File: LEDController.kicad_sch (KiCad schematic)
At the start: 15 parts, among them J1 3557-2, J11 TB002-500-04BE, J12 TB002-500-04BE, J16 3557-2, J17 TB002-500-04BE, J2 3557-2, J3 3557-2, J4 3557-2, J5 3557-2, J6 3557-2, J7 VP0265840000G, K1 J115F11CH5VDCS61.5U, Q1 BCX56,135

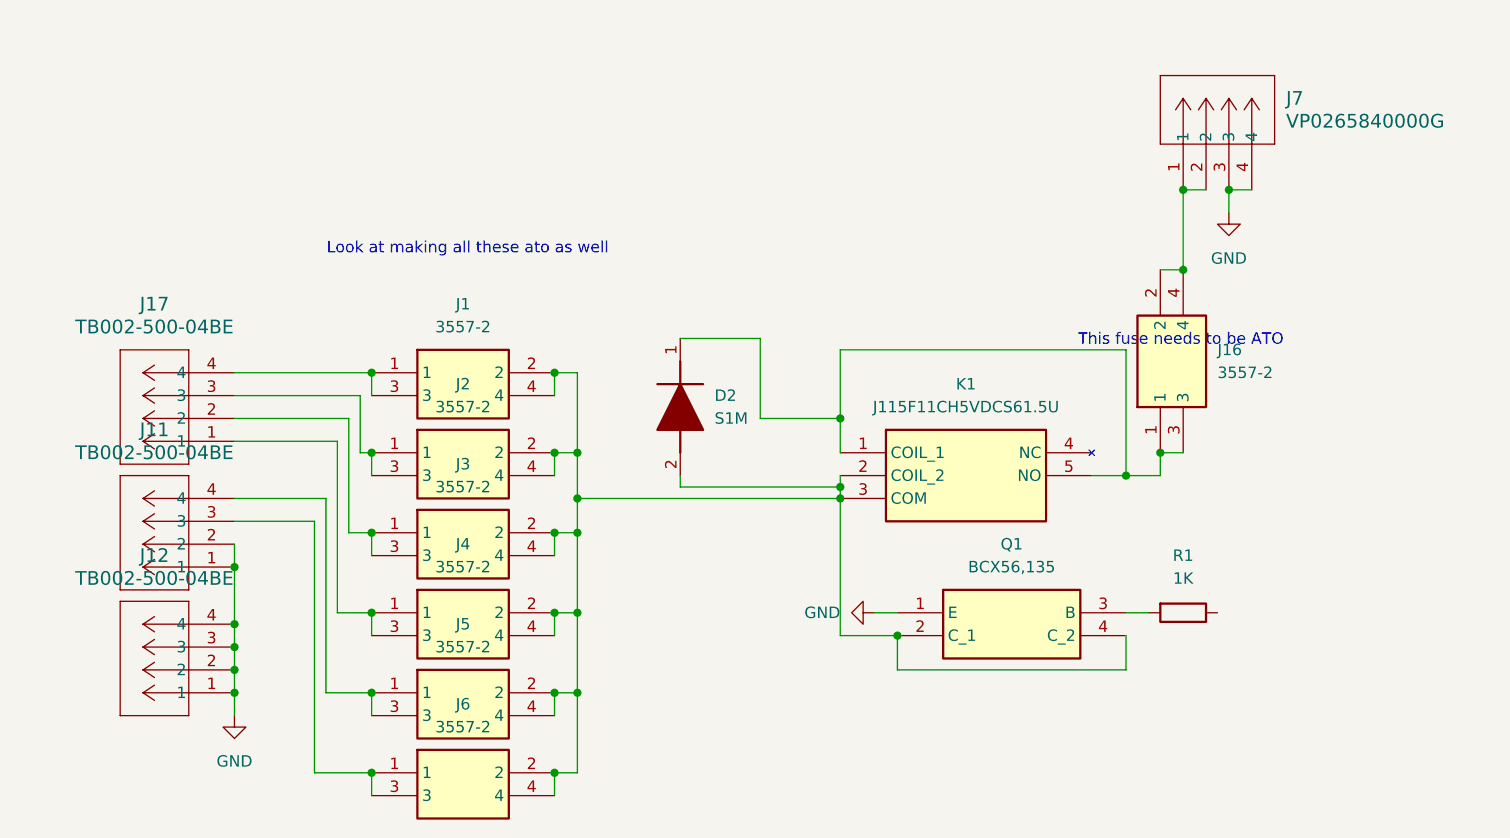
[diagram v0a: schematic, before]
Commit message: final schematic
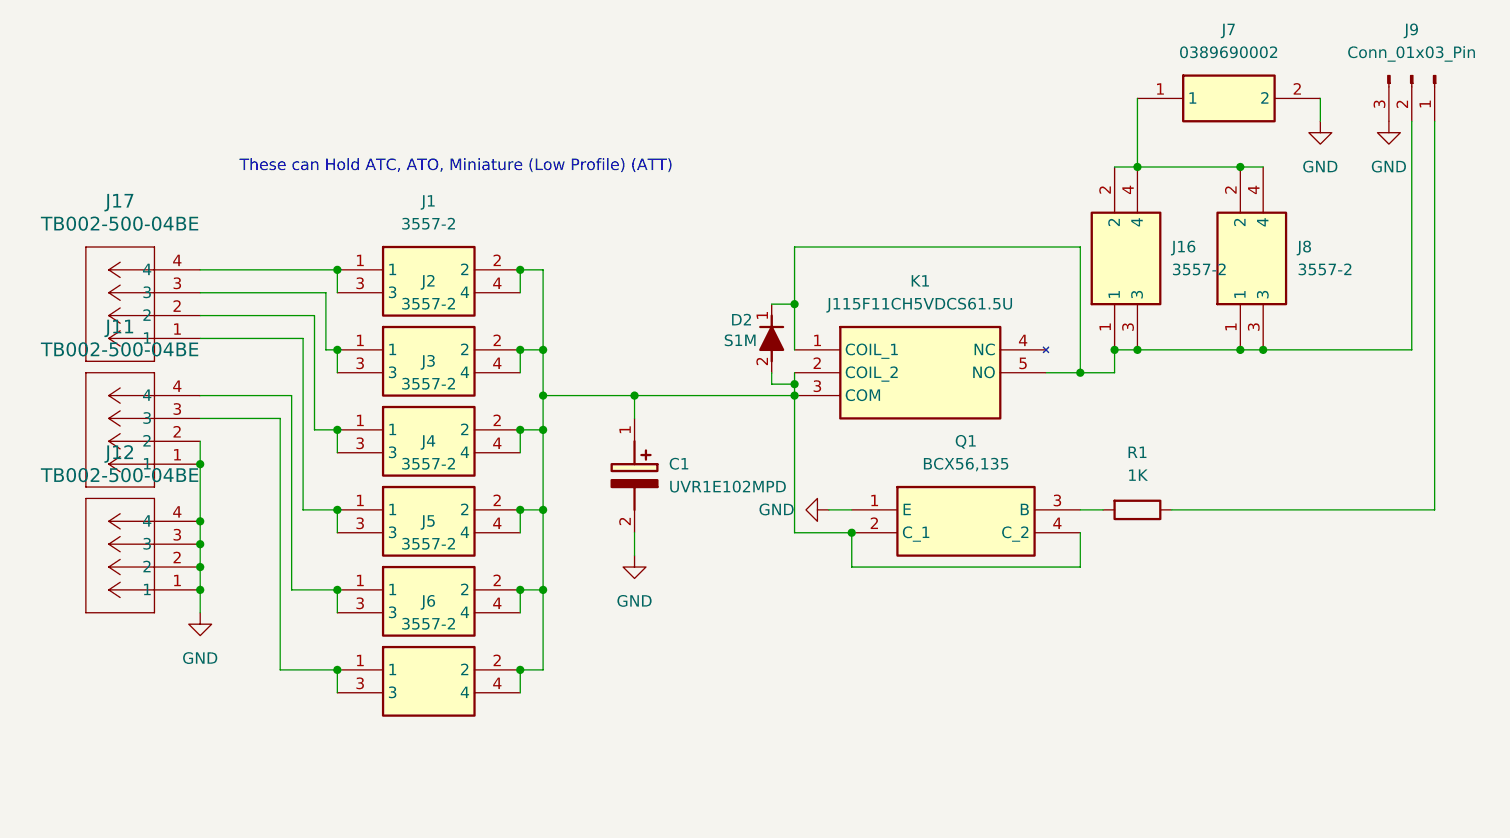
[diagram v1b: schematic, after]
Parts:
- removed J7: VP0265840000G, CONN04_VP026584_20P32X18P3_AMP, symbol SamacSys_Parts:VP0265840000G
- added C1: UVR1E102MPD, CAPPRD500W60D1025H2200, symbol SamacSys_Parts:UVR1E102MPD
- added J7: 0389690002, 0389690002, symbol SamacSys_Parts:0389690002
- added J8: 3557-2, 3557-2, symbol SamacSys_Parts:3557-2
- added J9: Conn_01x03_Pin, Connector_PinSocket_2.54mm:PinSocket_1x03_P2.54mm_Vertical, symbol Connector:Conn_01x03_Pin
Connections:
- net GND: now also C1.2 (-), J7.2, J9.3 (Pin_3)
- net at D2.2 (A), J1.2, J1.4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: now also C1.1 (+)
- net at D2.1 (K), J16.1, J16.3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: now also J8.1, J8.3, J9.2 (Pin_2)
- net at R1.1: now also J9.1 (Pin_1)
- net at J16.2, J16.4: now also J7.1, J8.2, J8.4
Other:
- note added: "These can Hold ATC, ATO, Miniature (Low Profile) (ATT)"
- note removed: "Look at making all these ato as well"
- note removed: "This fuse needs to be ATO"
- moved on the sheet: D2, J1, J11, J12, J16, J17, J2, J3, J4, J5, J6, K1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

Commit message: wip layout
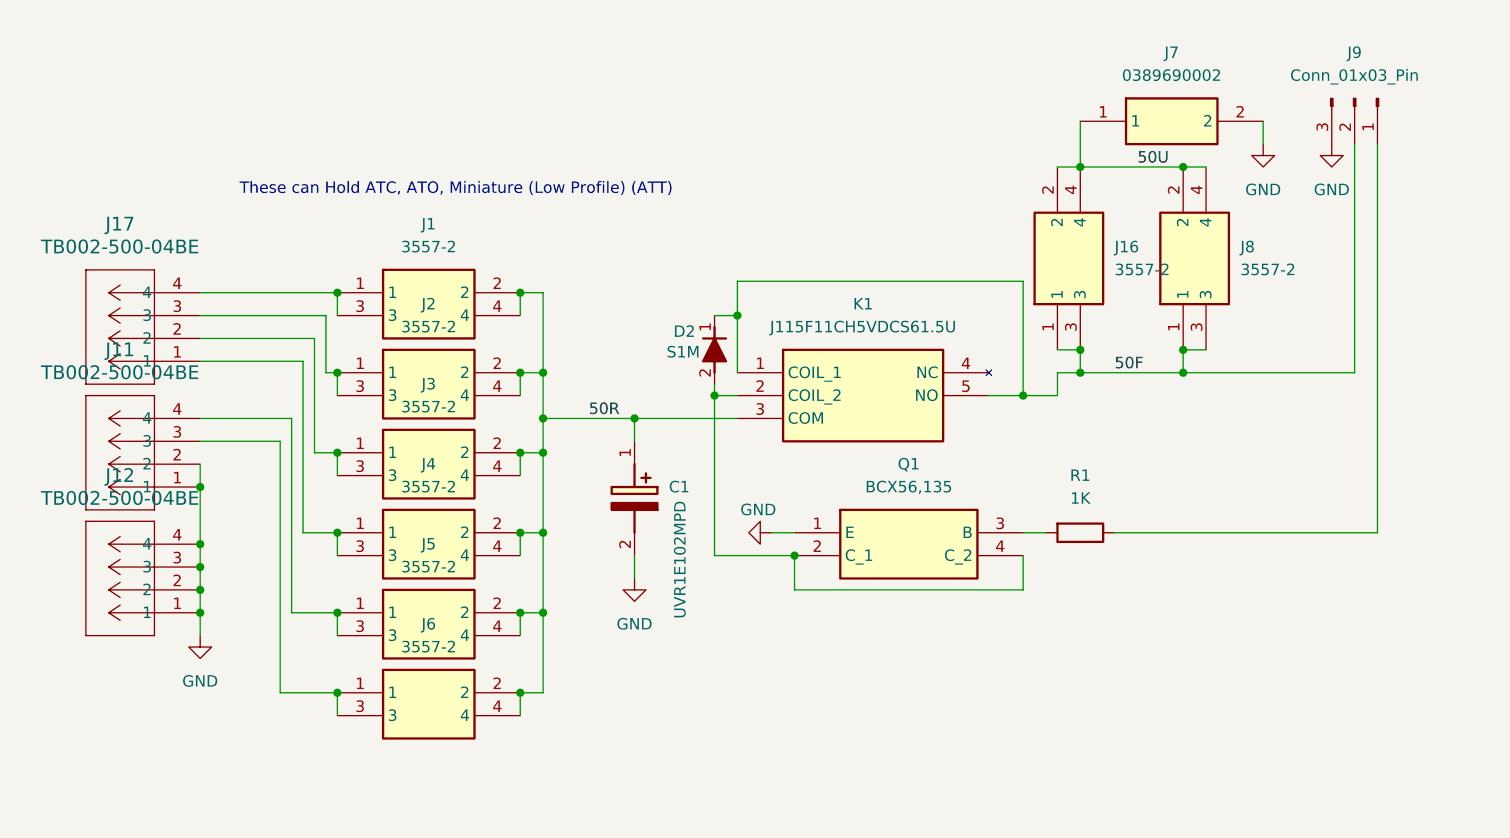
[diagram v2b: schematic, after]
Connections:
- net 50R: now reaches C1.1 (+), J1.2, J1.4, J2.2, J2.4, J3.2, J3.4, J4.2, J4.4, J5.2, J5.4, J6.2, J6.4, K1.3 (COM)
- net 50R: no longer D2.2 (A), K1.2 (COIL_2), Q1.2 (C_1), Q1.4 (C_2)
- net 50F: now reaches D2.1 (K), J16.1, J16.3, J8.1, J8.3, J9.2 (Pin_2), K1.1 (COIL_1), K1.5 (NO)
- net 50U: now reaches J16.2, J16.4, J7.1, J8.2, J8.4
- new net: D2.2 (A), K1.2 (COIL_2), Q1.2 (C_1), Q1.4 (C_2)
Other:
- moved on the sheet: C1, D2, J1, J11, J12, J16, J17, J2, J3, J4, J5, J6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
